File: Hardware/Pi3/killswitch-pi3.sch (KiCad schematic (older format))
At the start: 26 parts, among them J1 PWR_IN, J2 REMOTE, J3 PI, Q1 Q_PMOS_GSD, SW1 SW_Push, U1 TSDP341xx, U2 AZ1117-3.3, U3 ATTINY1634-SU

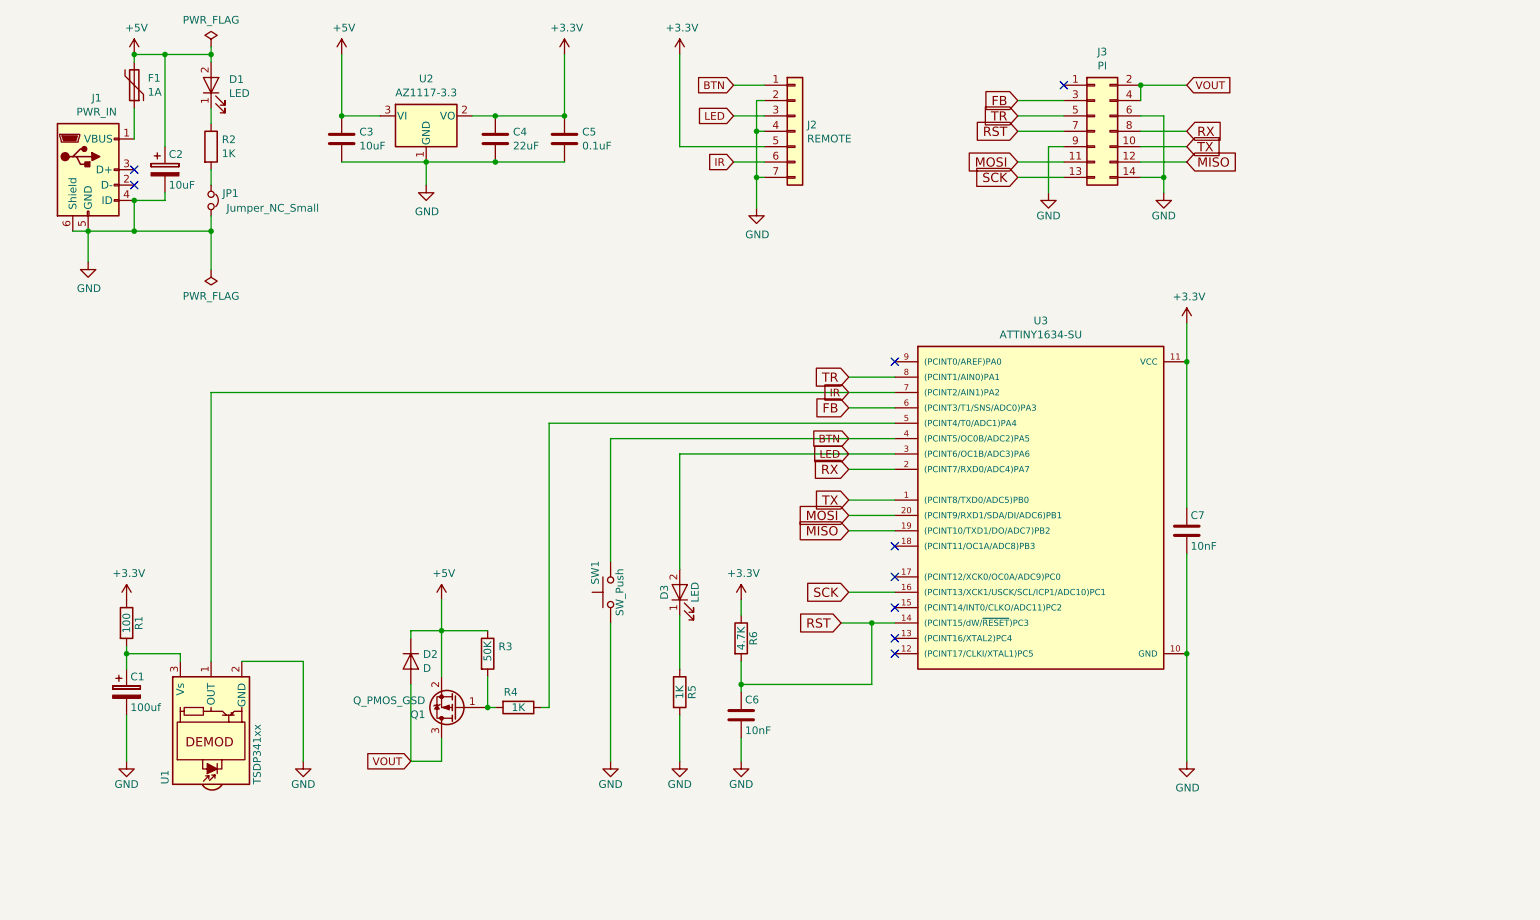
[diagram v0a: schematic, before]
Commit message: new schematic/pcb for 1634
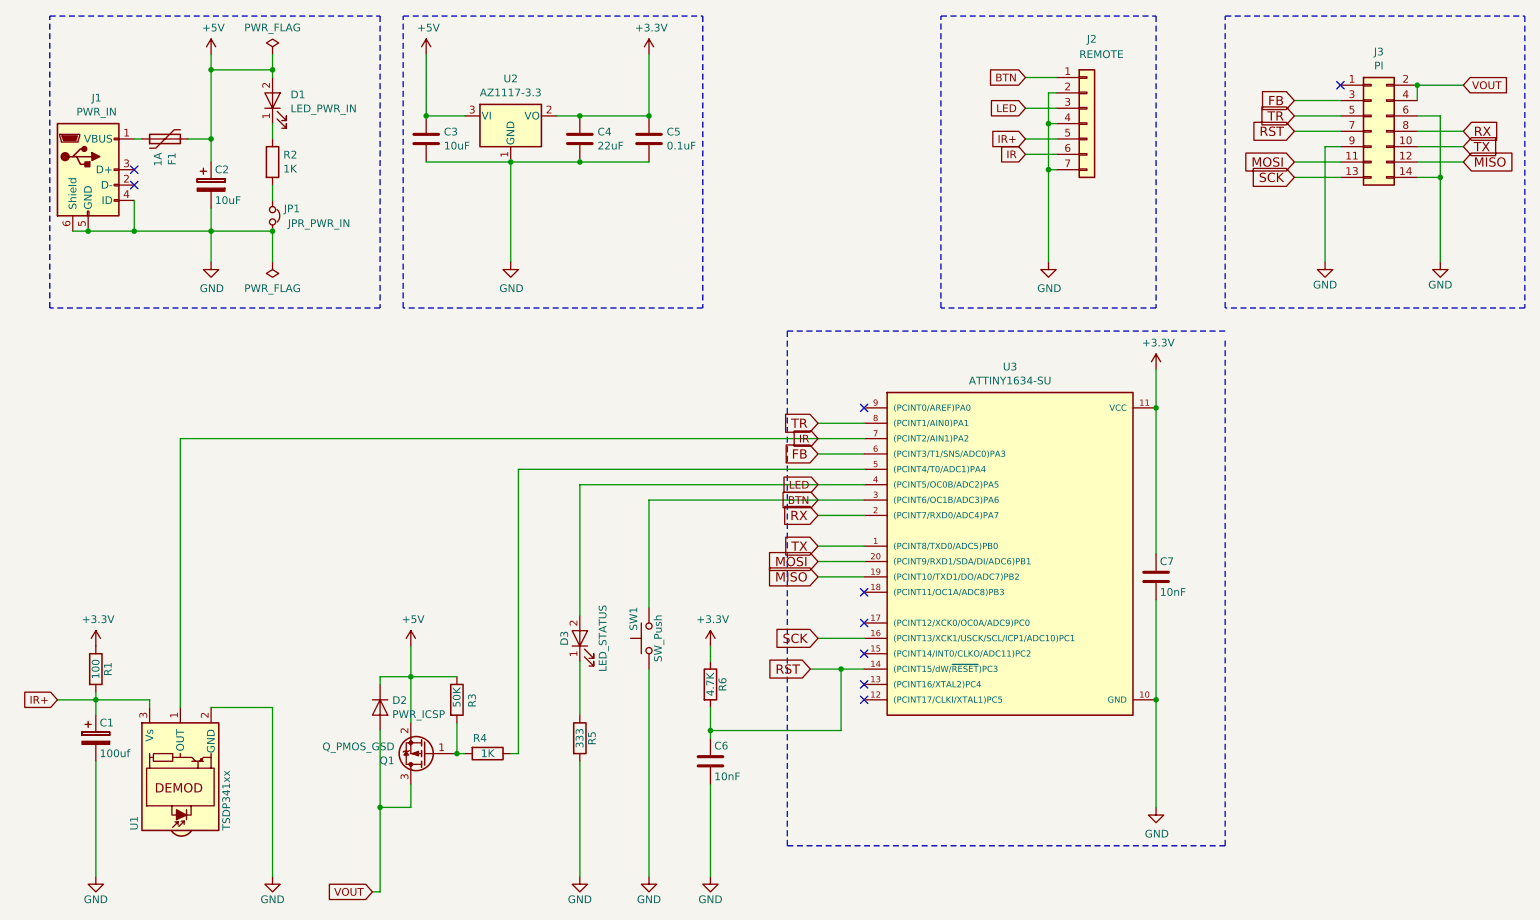
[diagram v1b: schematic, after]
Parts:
- D1: value LED -> LED_PWR_IN
- D2: value D -> PWR_ICSP
- D3: value LED -> LED_STATUS
- JP1: value Jumper_NC_Small -> JPR_PWR_IN
- R5: value 1K -> 333
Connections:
- net +3V3: no longer J2.5 (Pin_5)
- net BTN: now also U3.3 ((PCINT6/OC1B/ADC3)PA6); no longer U3.4 ((PCINT5/OC0B/ADC2)PA5)
- net LED: now also U3.4 ((PCINT5/OC0B/ADC2)PA5); no longer U3.3 ((PCINT6/OC1B/ADC3)PA6)
- net IR+: now reaches C1.1, R1.2, U1.3 (Vs)
- net IR+: now also J2.5 (Pin_5)
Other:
- moved on the sheet: C1, C2, C3, C4, C5, C6, C7, D1, D2, D3, F1, J2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
